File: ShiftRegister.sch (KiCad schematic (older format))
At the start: 1 part, among them U2 74HCT164

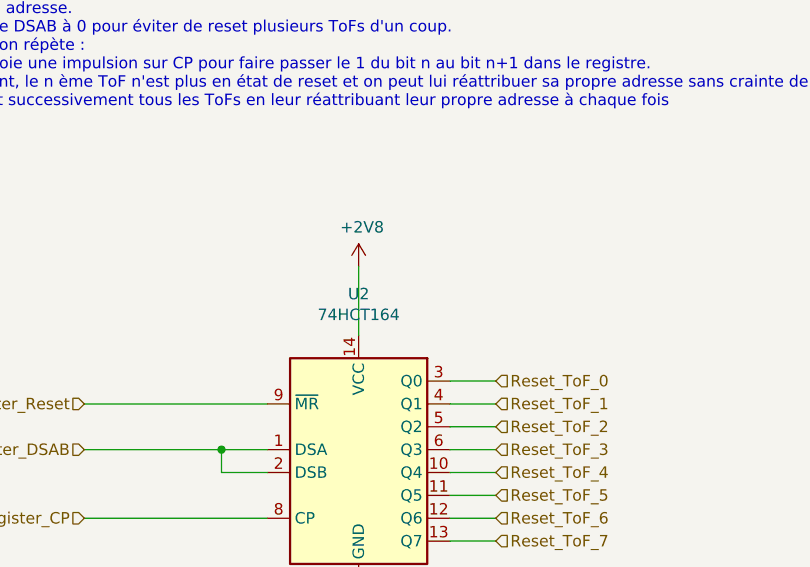
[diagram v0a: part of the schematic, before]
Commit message: Add files via upload
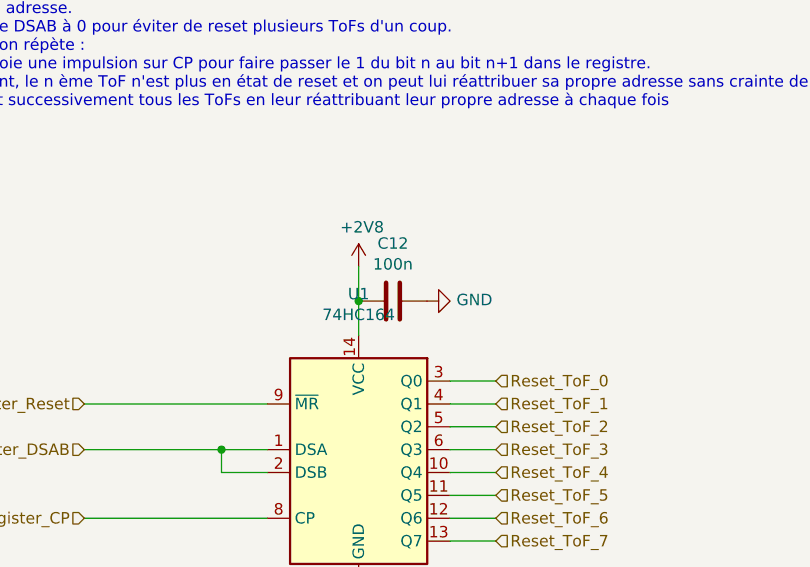
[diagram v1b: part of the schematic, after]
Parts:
- removed U2: 74HCT164, symbol 74xx:74HCT164
- added C12: 100n, symbol Device:C
- added U1: 74HC164, symbol 74xx:74HC164
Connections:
- net +2V8: now also C12.2, U1.14 (VCC)
- net GND: now also C12.1, U1.7 (GND)
- net Reset_ToF_0: now also U1.3 (Q0)
- net Reset_ToF_1: now also U1.4 (Q1)
- net Reset_ToF_2: now also U1.5 (Q2)
- net Reset_ToF_3: now also U1.6 (Q3)
- net Reset_ToF_4: now also U1.10 (Q4)
- net Reset_ToF_5: now also U1.11 (Q5)
- net Reset_ToF_6: now also U1.12 (Q6)
- net Reset_ToF_7: now also U1.13 (Q7)
- net ShiftRegister_CP: now also U1.8 (CP)
- net ShiftRegister_DSAB: now also U1.1 (DSA), U1.2 (DSB)
- net ShiftRegister_Reset: now also U1.9 (~MR)
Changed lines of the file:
@@
 $Descr A4 11693 8268
 encoding utf-8
-Sheet 11 23
+Sheet 11 22
 Title ""
 Date ""
@@
 Text HLabel 6650 3450 2    50   Input ~ 0
 Reset_ToF_0
-$Comp
-L 74xx:74HCT164 U2
-U 1 1 5E67260D
-P 6050 3750
-F 0 "U2" H 6050 4431 50  0000 C CNN
-F 1 "74HCT164" H 6050 4340 50  0000 C CNN
-F 2 "" H 6950 3450 50  0001 C CNN
-F 3 "https://assets.nexperia.com/documents/data-sheet/74HC_HCT164.pdf" H 6950 3450 50  0001 C CNN
-	1    6050 3750
-	1    0    0    -1
-$EndComp
 Text HLabel 4850 3550 0    50   Input ~ 0
 ShiftRegister_Reset
@@
 	1    0    0    -1
 $EndComp
-Wire Wire Line
-	6050 2950 6050 3250
 $Comp
 L power:+2V8 #PWR022
@@
 Text Notes 4200 2500 0    50   ~ 0
 Registre à décalage :\nà cause de la configuration interne des ToFs, il n'est pas possible de les reset tous en même temps car alors les adresses I2C se \nréattribueraient un peu n'importe comment et ne \npermettraient plus au microcontrôleur de savoir quel ToF a \nquelle adresse. \nC'est pourquoi on a choisi d'utiliser un registre à décalage : \nLorqsqu'il faut reset les ToFs, on passe DSAB à 1 puis on envoie une impulsion sur CP pour mettre ce 1 dans le premier bit du registre.\nCeci aura pour effet de reset le premier ToF qui ne connaît alors\nplus son adresse.\nOn passe DSAB à 0 pour éviter de reset plusieurs ToFs d'un coup.\nEnsuite on répète :\n"On envoie une impulsion sur CP pour faire passer le 1 du bit n au bit n+1 dans le registre.\nCe faisant, le n ème ToF n'est plus en état de reset et on peut lui réattribuer sa propre adresse sans crainte de confusion."\nOn reset successivement tous les ToFs en leur réattribuant leur propre adresse à chaque fois\n\n\n\n
+$Comp
+L 74xx:74HC164 U1
+U 1 1 5E7FC43F
+P 6050 3750
+F 0 "U1" H 6050 4431 50  0000 C CNN
+F 1 "74HC164" H 6050 4340 50  0000 C CNN
+F 2 "" H 6950 3450 50  0001 C CNN
+F 3 "https://assets.nexperia.com/documents/data-sheet/74HC_HCT164.pdf" H 6950 3450 50  0001 C CNN
+	1    6050 3750
+	1    0    0    -1
+$EndComp
+Wire Wire Line
+	6050 2950 6050 3100
+$Comp
+L Device:C C12
+U 1 1 5E832490
+P 6200 3100
+F 0 "C12" V 5948 3100 50  0000 C CNN
+F 1 "100n" V 6039 3100 50  0000 C CNN
+F 2 "" H 6238 2950 50  0001 C CNN
+F 3 "~" H 6200 3100 50  0001 C CNN
+	1    6200 3100
+	0    1    1    0
+$EndComp
+Connection ~ 6050 3100
+Wire Wire Line
+	6050 3100 6050 3250
+$Comp
+L power:GND #PWR0116
+U 1 1 5E833001
+P 6350 3100
+F 0 "#PWR0116" H 6350 2850 50  0001 C CNN
+F 1 "GND" V 6355 2972 50  0000 R CNN
+F 2 "" H 6350 3100 50  0001 C CNN
+F 3 "" H 6350 3100 50  0001 C CNN
+	1    6350 3100
+	0    -1   -1   0
+$EndComp
 $EndSCHEMATC

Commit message: Add files via upload
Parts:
- C12: footprint (none) -> Capacitor_SMD:C_0805_2012Metric_Pad1.15x1.40mm_HandSolder
- U1: footprint (none) -> Package_SO:SOIC-14_3.9x8.7mm_P1.27mm
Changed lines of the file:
@@
 EESchema Schematic File Version 4
-LIBS:kicad_master-cache
 EELAYER 30 0
 EELAYER END
 $Descr A4 11693 8268
 encoding utf-8
-Sheet 11 22
+Sheet 11 21
 Title ""
 Date ""
@@
 F 0 "U1" H 6050 4431 50  0000 C CNN
 F 1 "74HC164" H 6050 4340 50  0000 C CNN
-F 2 "" H 6950 3450 50  0001 C CNN
+F 2 "Package_SO:SOIC-14_3.9x8.7mm_P1.27mm" H 6950 3450 50  0001 C CNN
 F 3 "https://assets.nexperia.com/documents/data-sheet/74HC_HCT164.pdf" H 6950 3450 50  0001 C CNN
 	1    6050 3750
@@
 F 0 "C12" V 5948 3100 50  0000 C CNN
 F 1 "100n" V 6039 3100 50  0000 C CNN
-F 2 "" H 6238 2950 50  0001 C CNN
+F 2 "Capacitor_SMD:C_0805_2012Metric_Pad1.15x1.40mm_HandSolder" H 6238 2950 50  0001 C CNN
 F 3 "~" H 6200 3100 50  0001 C CNN
 	1    6200 3100

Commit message: avancement général du routage
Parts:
- C12: symbol Device:C -> shield_etage2-rescue:C-Device
- U1: symbol 74xx:74HC164 -> shield_etage2-rescue:74HC164-74xx
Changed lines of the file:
@@
 	5650 4050 4850 4050
 $Comp
-L power:GND #PWR023
+L shield_etage2-rescue:GND-power #PWR023
 U 1 1 5E67AFE4
 P 6050 4350
@@
 $EndComp
 $Comp
-L power:+2V8 #PWR022
+L shield_etage2-rescue:+2V8-power #PWR022
 U 1 1 5E67E563
 P 6050 2950
@@
 Registre à décalage :\nà cause de la configuration interne des ToFs, il n'est pas possible de les reset tous en même temps car alors les adresses I2C se \nréattribueraient un peu n'importe comment et ne \npermettraient plus au microcontrôleur de savoir quel ToF a \nquelle adresse. \nC'est pourquoi on a choisi d'utiliser un registre à décalage : \nLorqsqu'il faut reset les ToFs, on passe DSAB à 1 puis on envoie une impulsion sur CP pour mettre ce 1 dans le premier bit du registre.\nCeci aura pour effet de reset le premier ToF qui ne connaît alors\nplus son adresse.\nOn passe DSAB à 0 pour éviter de reset plusieurs ToFs d'un coup.\nEnsuite on répète :\n"On envoie une impulsion sur CP pour faire passer le 1 du bit n au bit n+1 dans le registre.\nCe faisant, le n ème ToF n'est plus en état de reset et on peut lui réattribuer sa propre adresse sans crainte de confusion."\nOn reset successivement tous les ToFs en leur réattribuant leur propre adresse à chaque fois\n\n\n\n
 $Comp
-L 74xx:74HC164 U1
+L shield_etage2-rescue:74HC164-74xx U1
 U 1 1 5E7FC43F
 P 6050 3750
+AR Path="/5E7FC43F" Ref="U1"  Part="1"
+AR Path="/5E627338/5E7FC43F" Ref="U1"  Part="1"
 F 0 "U1" H 6050 4431 50  0000 C CNN
 F 1 "74HC164" H 6050 4340 50  0000 C CNN
@@
 	6050 2950 6050 3100
 $Comp
-L Device:C C12
+L shield_etage2-rescue:C-Device C12
 U 1 1 5E832490
 P 6200 3100
@@
 	6050 3100 6050 3250
 $Comp
-L power:GND #PWR0116
+L shield_etage2-rescue:GND-power #PWR0116
 U 1 1 5E833001
 P 6350 3100
